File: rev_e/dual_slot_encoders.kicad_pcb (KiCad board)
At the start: 2 copper layers, 50 x 25 mm, 14 parts, among them U1 GP1S094HCZ0F, U2 GP1S094HCZ0F, U3 GPS1S97HCZ0F, U4 GPS1S97HCZ0F

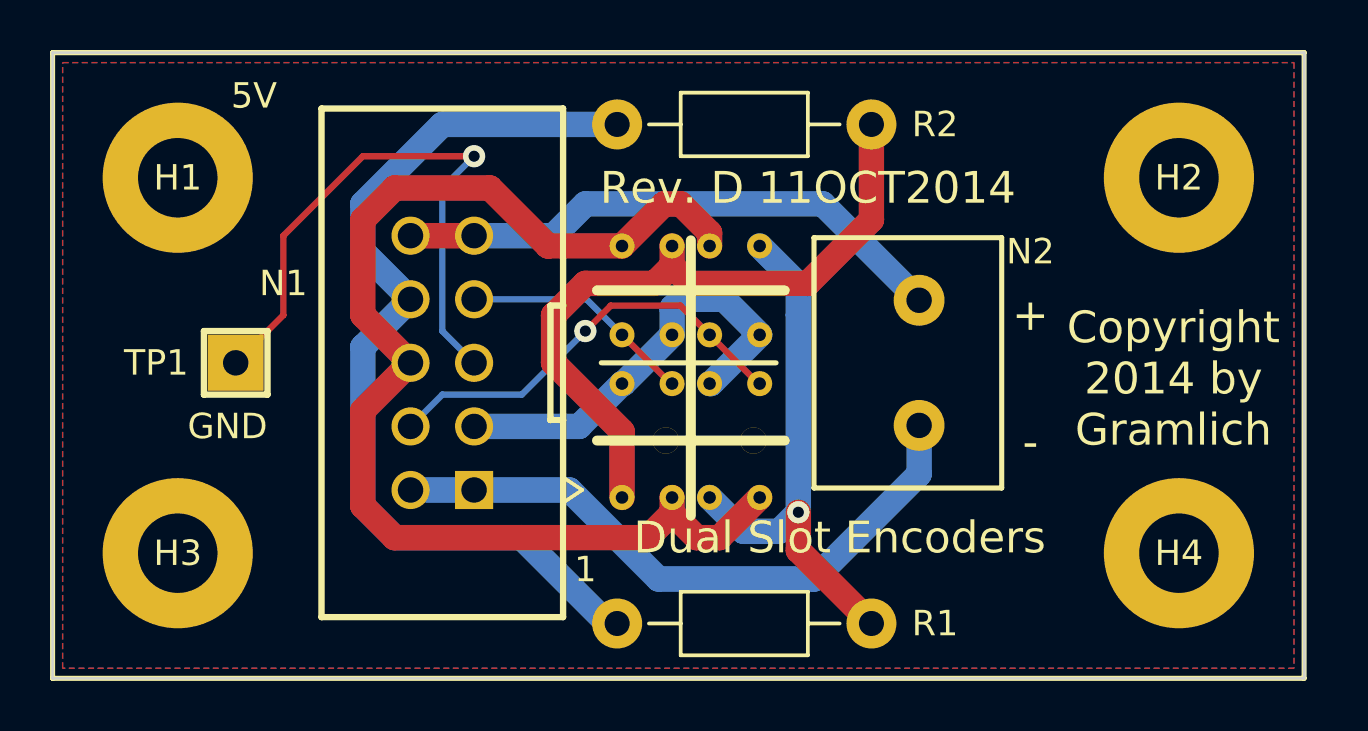
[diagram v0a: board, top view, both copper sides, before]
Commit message: Got Rev. E wrapped up.
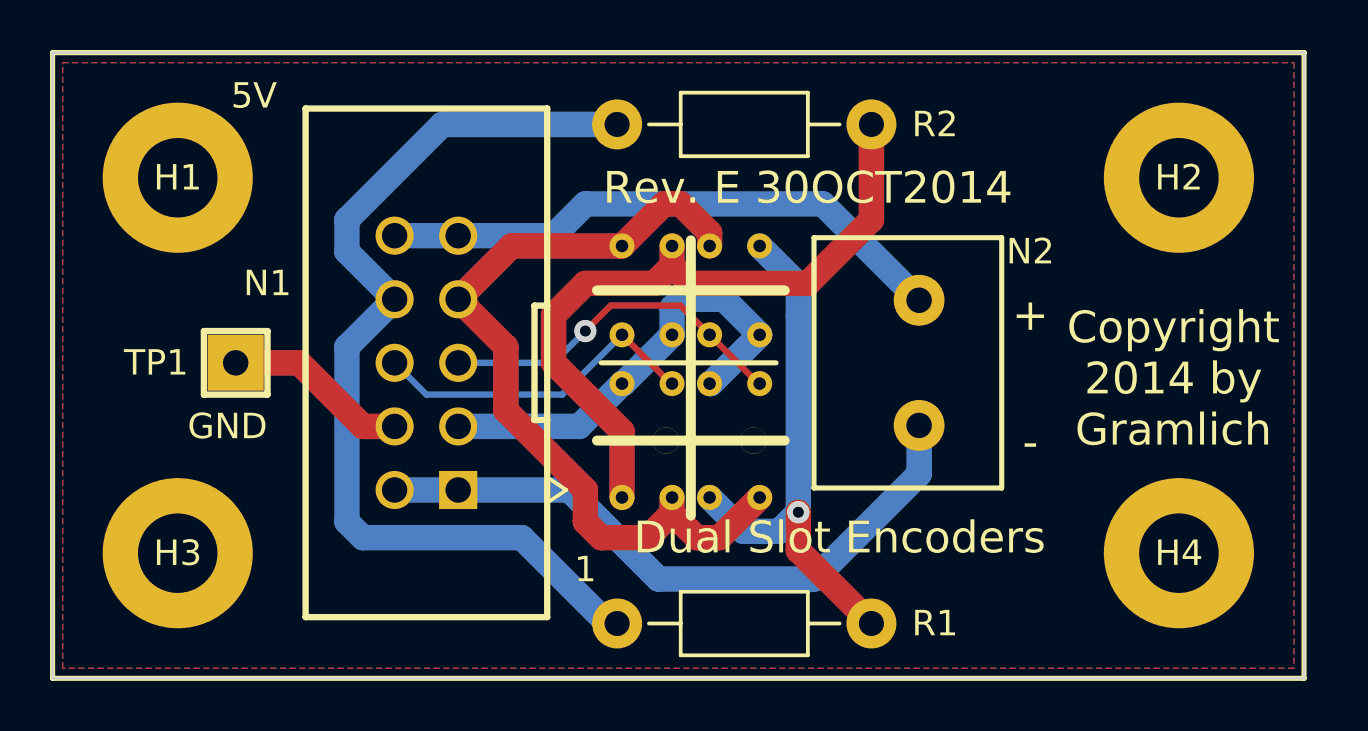
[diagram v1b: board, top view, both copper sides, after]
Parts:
- moved N1 0.63 mm to (114.9, 112.4)
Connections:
- N1 pad 4: /A -> /LGND
- N1 pad 5: /LGND -> /A
- N1 pad 6: /LED_EN -> /B
- N1 pad 7: /B -> /LED_EN
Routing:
- net /LGND: track 24.1 -> 7.42 mm, vias 1 -> 0
- net /LED_EN: track 48.5 -> 33.0 mm
- net /B: track 9.31 -> 13.4 mm
- net /A: track 17.2 -> 14.3 mm
- net /BPWR: track 37.2 -> 38.5 mm
- net /LPWR: track 18.0 -> 18.6 mm
- net /MOTOR-: track 22.4 -> 23.1 mm
- net /MOTOR+: track 25.5 -> 26.1 mm
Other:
- board text added: "Rev. E 30OCT2014"
- board text removed: "Rev. D 11OCT2014"
